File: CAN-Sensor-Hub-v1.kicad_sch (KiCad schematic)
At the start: 62 parts, among them J1 Conn_01x04, J10 Conn_01x03, J11 Conn_01x03, J2 Conn_01x04, J3 Conn_01x04, J4 USB_C_Receptacle_USB2.0_14P, J5 Conn_ARM_JTAG_SWD_10, J6 Conn_01x04, J7 Conn_01x04, J8 Conn_01x04, J9 Conn_01x03, Q1 NMOS, Q2 NMOS, Q3 PMOS, SW1 NRST, SW2 BOOT, U1 TPS5430DDA, U2 TCAN1042DRQ1, U3 W25Q32JVZP, U4 AZ1117-3.3, U7 STM32F722VETx, X1 8MHz, X2 32.768KHz

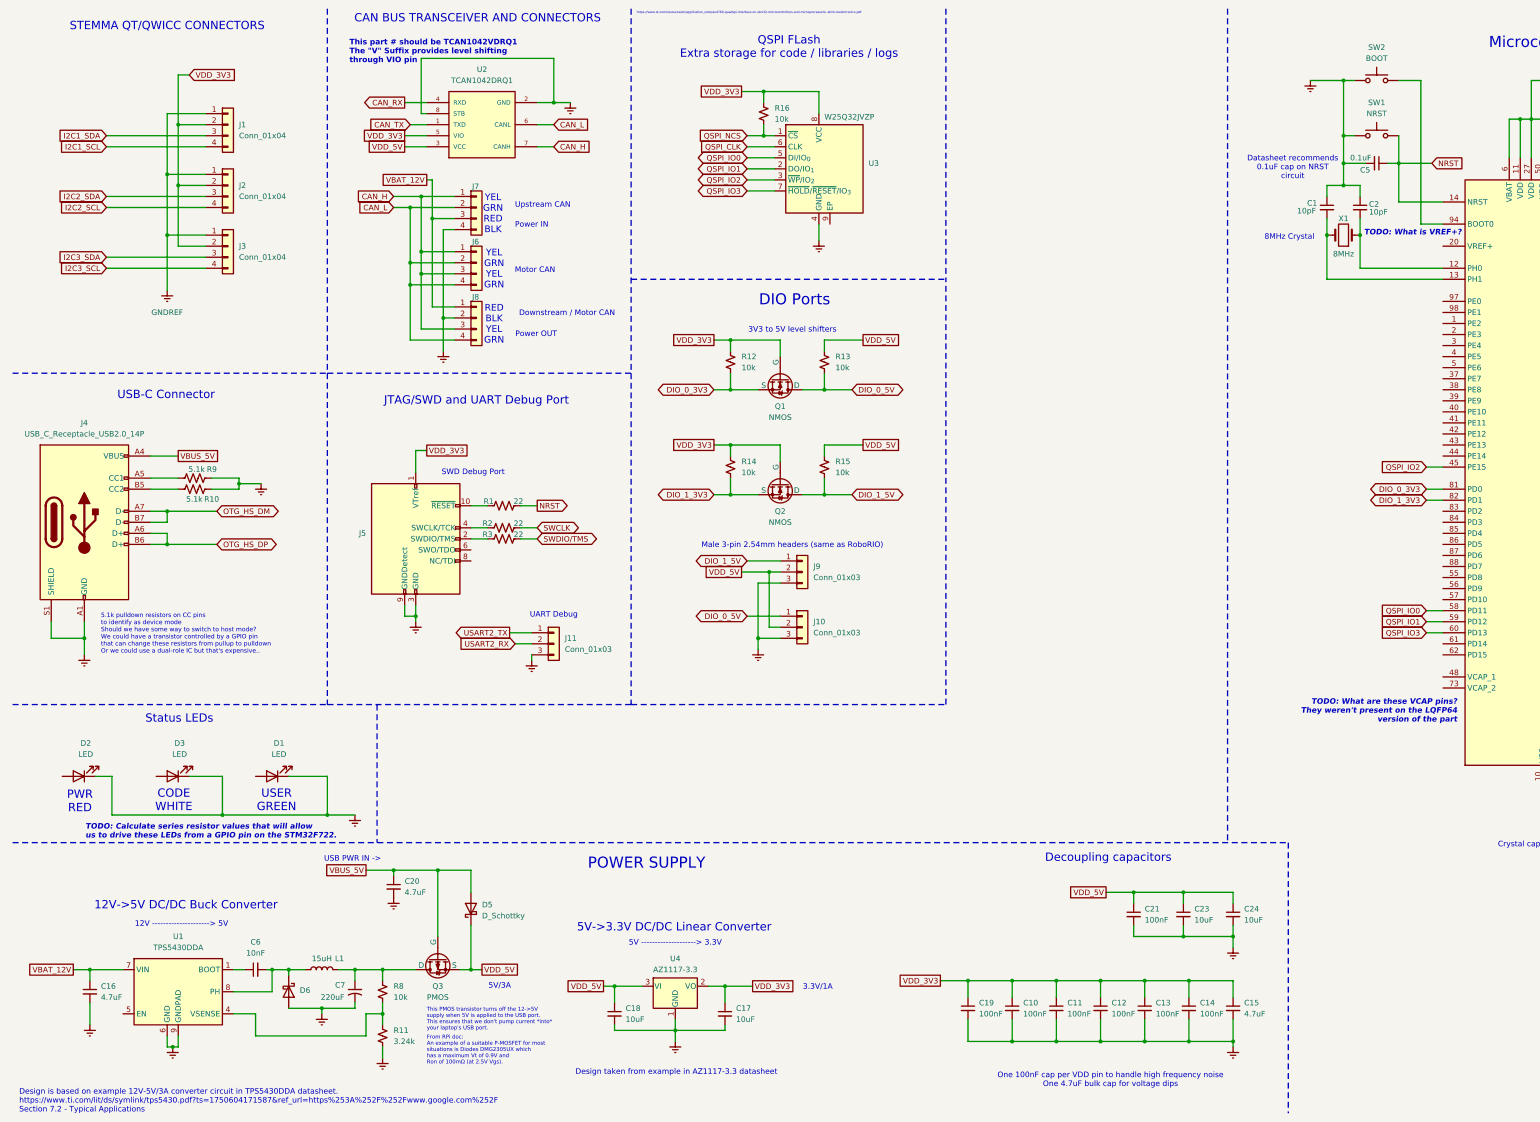
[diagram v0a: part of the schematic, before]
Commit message: V0.2 of board, nearly ready for production
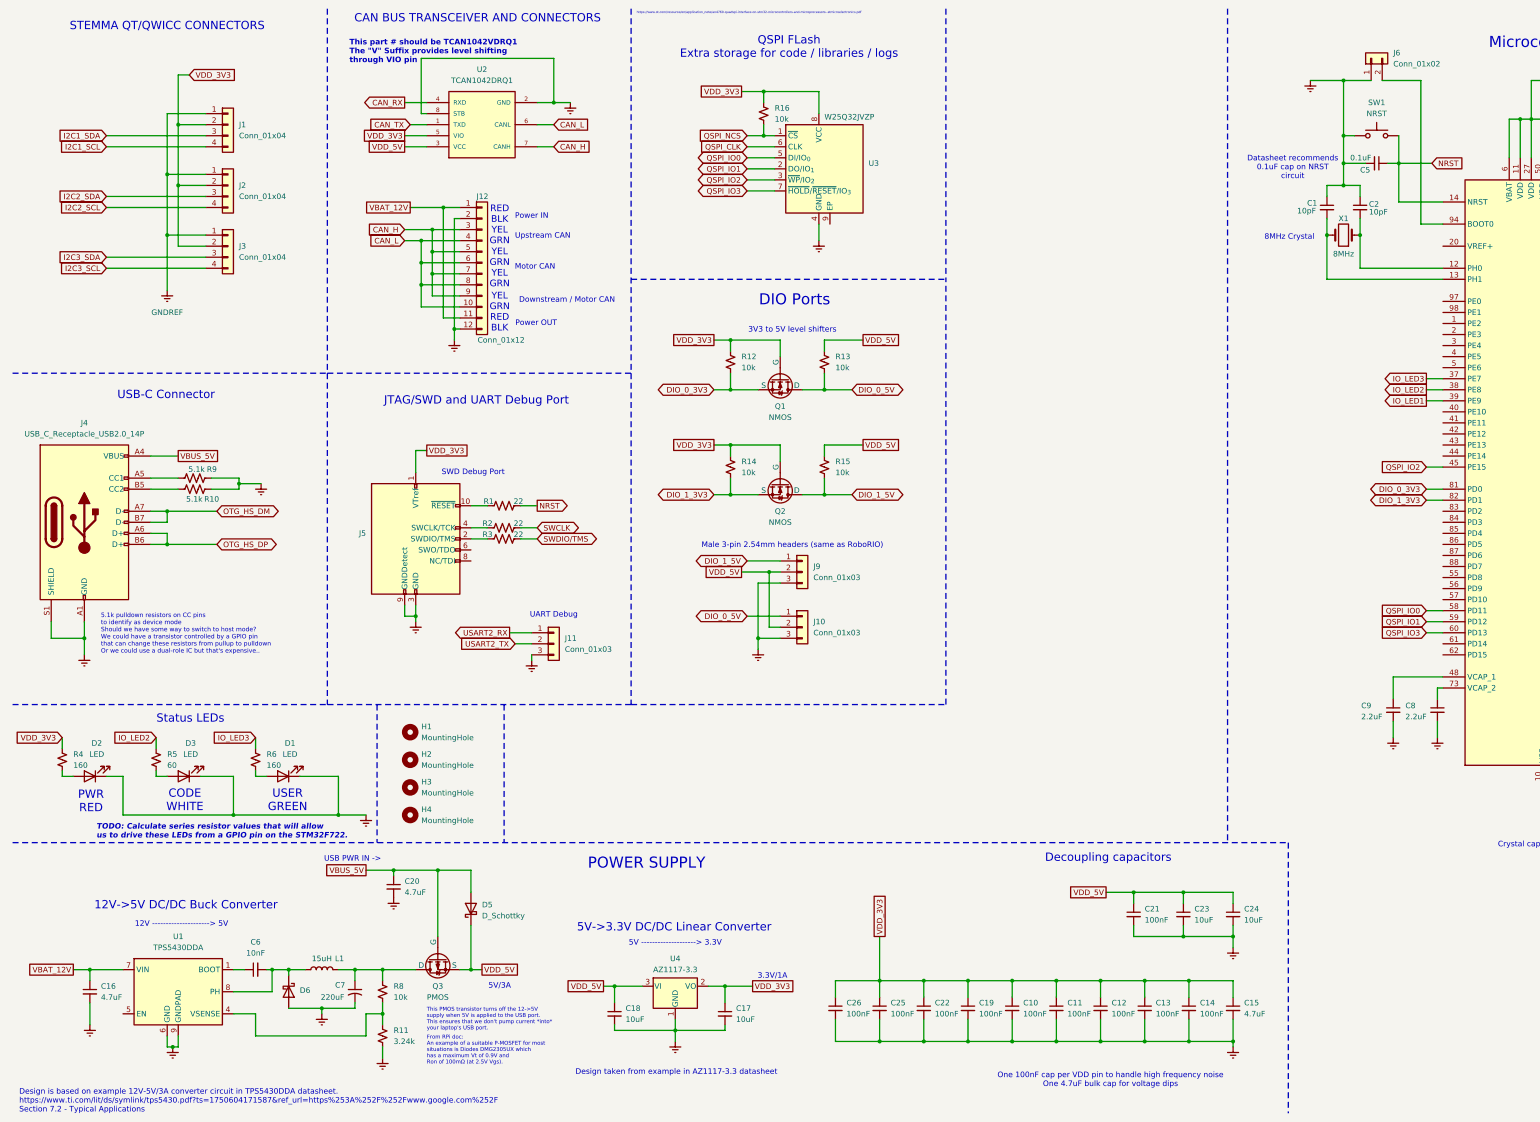
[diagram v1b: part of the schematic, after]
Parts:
- removed J6, J7, J8: Conn_01x04, TerminalBlock_WAGO:TerminalBlock_WAGO_2601-1104_1x04_P3.50mm_Horizontal, symbol Connector_Generic:Conn_01x04
- removed SW2: BOOT, lib:SW_TS-1088-AR02016, symbol Switch:SW_Push
- added C22, C25, C26: 100nF, Capacitor_SMD:C_0402_1005Metric, symbol Device:C_Small
- added C8, C9: 2.2uF, Capacitor_SMD:C_0402_1005Metric, symbol Device:C_Small
- added H1, H2, H3, H4: MountingHole, MountingHole:MountingHole_2.7mm_M2.5, symbol Mechanical:MountingHole
- added J12: Conn_01x12, TerminalBlock_WAGO:TerminalBlock_WAGO_2601-1112_1x12_P3.50mm_Horizontal, symbol Connector_Generic:Conn_01x12
- added J6: Conn_01x02, Connector_PinHeader_2.54mm:PinHeader_1x02_P2.54mm_Vertical, symbol Connector_Generic:Conn_01x02
- added R4, R6: 160, Resistor_SMD:R_0402_1005Metric, symbol Device:R_Small_US
- added R5: 60, Resistor_SMD:R_0402_1005Metric, symbol Device:R_Small_US
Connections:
- net CAN_H: now also J12.3 (Pin_3), J12.5 (Pin_5), J12.7 (Pin_7), J12.9 (Pin_9)
- net CAN_L: now also J12.10 (Pin_10), J12.4 (Pin_4), J12.6 (Pin_6), J12.8 (Pin_8)
- net GNDREF: now also C22.2, C25.2, C26.2, C8.2, C9.2, J12.12 (Pin_12), J12.2 (Pin_2), J6.1 (Pin_1)
- net USART2_RX: now also J11.1 (Pin_1); no longer J11.2 (Pin_2)
- net USART2_TX: now also J11.2 (Pin_2); no longer J11.1 (Pin_1)
- net VBAT_12V: now also J12.1 (Pin_1), J12.11 (Pin_11)
- net VDD_3V3: now also C22.1, C25.1, C26.1, R4.1
- net at D3.2 (A): now also R5.2
- net IO_LED3: now reaches U7.37 (PE7)
- net IO_LED3: now also R6.1
- net IO_LED2: now reaches U7.38 (PE8)
- net IO_LED2: now also R5.1
- net IO_LED1: now reaches U7.39 (PE9)
- net at U7.48 (VCAP_1): now also C9.1
- net at U7.73 (VCAP_2): now also C8.1
- net at U7.94 (BOOT0): now also J6.2 (Pin_2)
- net at D1.2 (A): now also R6.2
- net at D2.2 (A): now also R4.2
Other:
- note removed: "TODO: What are these VCAP pins? They weren't present on the LQFP64 version of the part"
- note removed: "TODO: What is VREF+?"
- moved on the sheet: D1, D2, D3
